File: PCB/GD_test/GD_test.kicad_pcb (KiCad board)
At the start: 2 copper layers, 46 x 51.3 mm, 47 parts, among them J1 RF_IN, J2 RF_IN, J3 RF_IN, J4 RF_IN, J5 Conn_01x01_Pin, J6 Conn_01x01_Pin, Q1 EPC2051, Q2 EPC2051, Q3 GS61004B-MR, Q5 EPC2014C, U1 LMG1020YFF, U10 TLV3501, U11 LMG1020YFF, U2 TLV3501, U3 NC7WZ04, U4 TLV3501, U5 NC7WZ04, U6 NC7WZ04, U7 NC7WZ04, U8 TLV3501, U9 LMG1020YFF

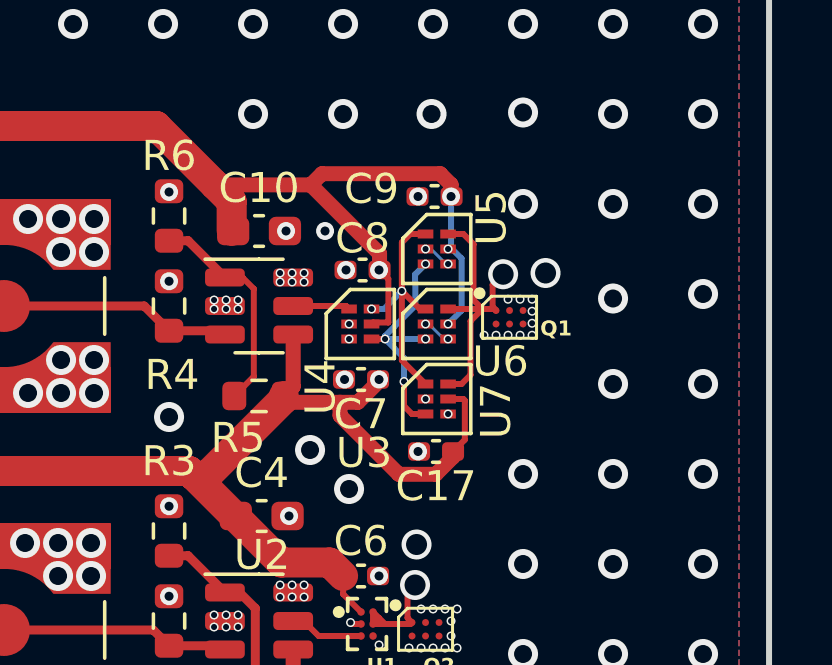
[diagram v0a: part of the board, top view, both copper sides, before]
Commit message: gate driver testboard rev 3 stuff
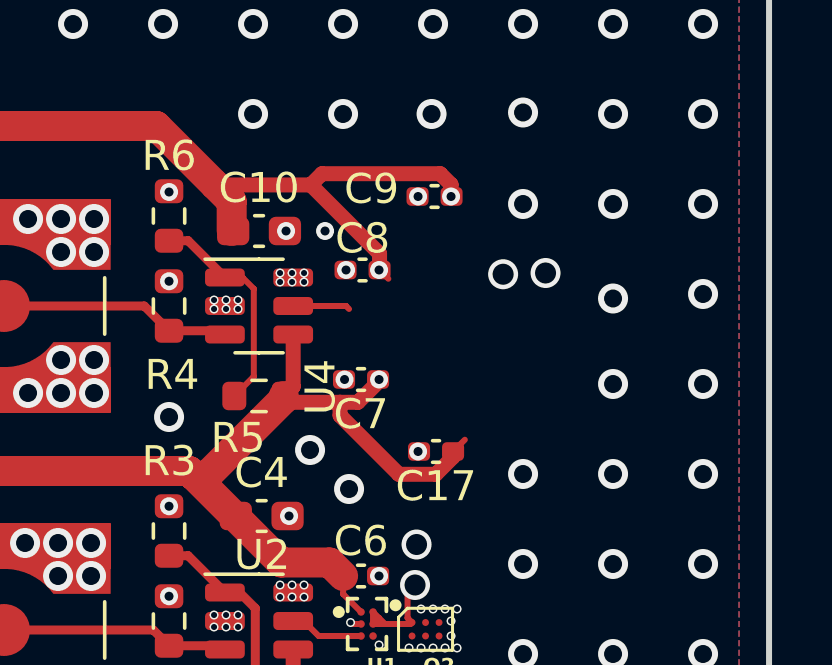
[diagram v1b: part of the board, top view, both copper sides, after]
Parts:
- removed Q1: EPC2051, EPCGaN:BGA-6_3x2_6.0x6.0mm
- removed U3, U5, U6, U7: NC7WZ04, pcbparts:SOIC-6
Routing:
- net Net-(Q1-G): track 9.54 -> 0.00 mm
- net +5V: track 186.2 -> 177.6 mm, vias 5 -> 3
- net /BUFF_OUT-: track 8.34 -> 0.00 mm, vias 4 -> 0
- net /BUFF_OUT+: track 8.25 -> 0.00 mm, vias 2 -> 0
- net GND: track 3.39 -> 1.47 mm, vias 368 -> 350

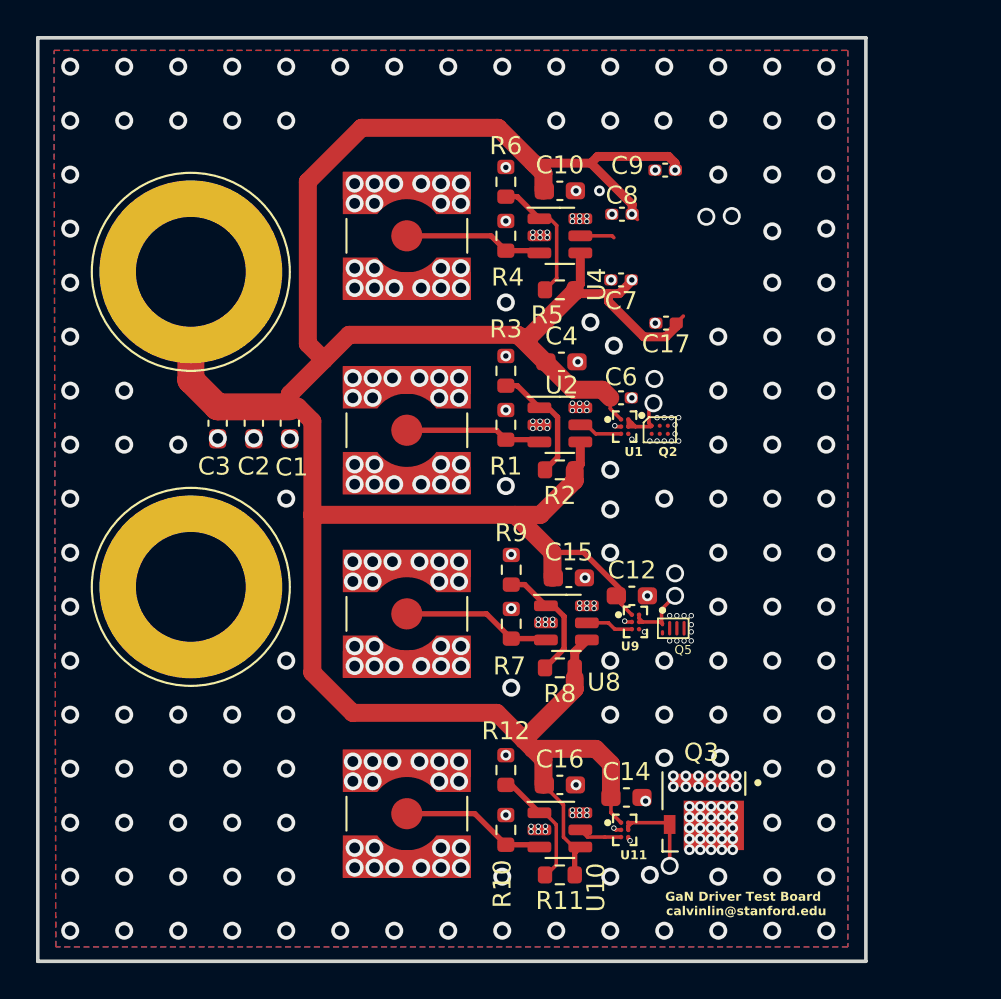
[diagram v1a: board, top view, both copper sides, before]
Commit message: gate driver test board rev 2 gerbers commit
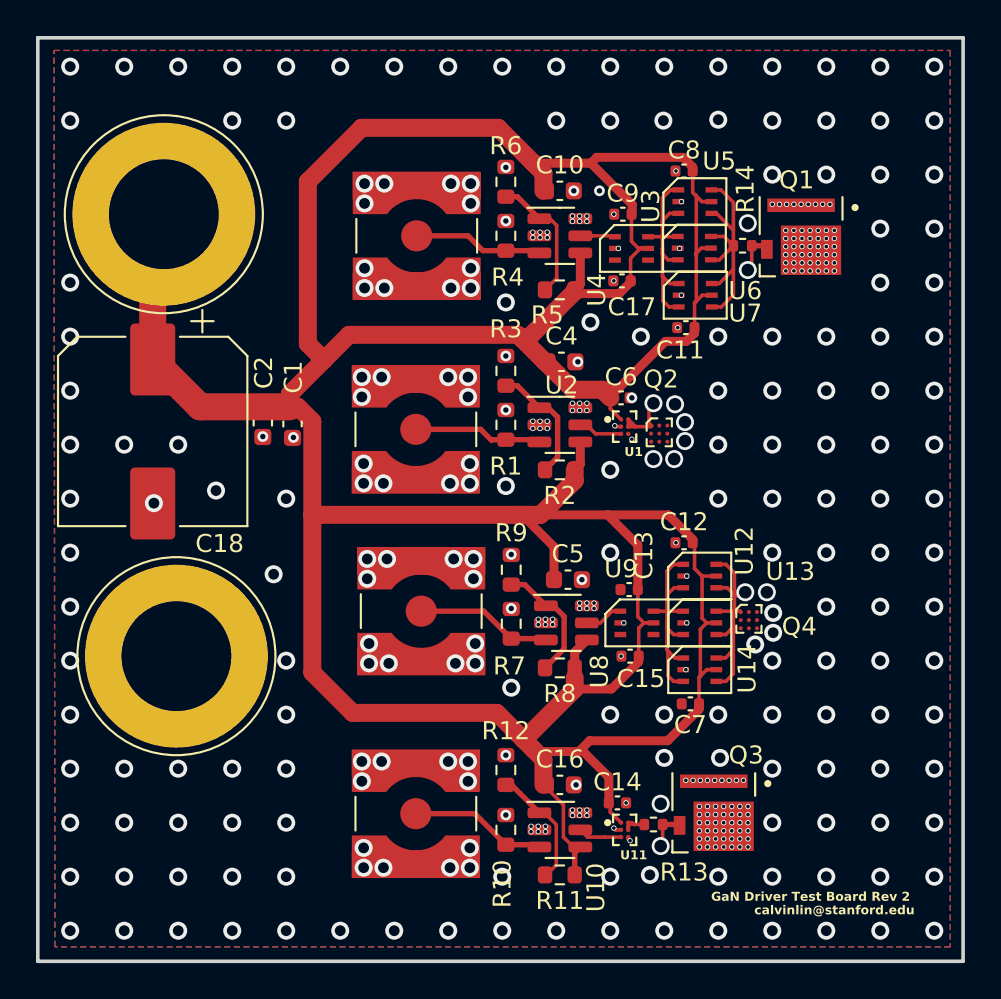
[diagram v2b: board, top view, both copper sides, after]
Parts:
- removed C3: C_Small, Capacitor_SMD:C_0603_1608Metric_Pad1.08x0.95mm_HandSolder
- removed Q5: EPC2014C, EPCGaN:EPC2014C
- added C11: C_Small, Capacitor_SMD:C_0402_1005Metric, F.Cu at (139.0, 81.6)
- added C13: C_Small, Capacitor_SMD:C_0402_1005Metric, F.Cu at (135.8, 96.2)
- added C18: C_Small, Capacitor_SMD:CP_Elec_10x10, F.Cu at (109.4, 87.4)
- added C5: C_Small, Capacitor_SMD:C_0603_1608Metric, F.Cu at (132.4, 95.6)
- added Q1: GS61004B-MR, EPCGaN:TRANS_GS61004B-MR, F.Cu at (145.4, 76.5)
- added Q4: EPC2214, pcbparts:BGA-9_3x3_6.0x6.0mm, F.Cu at (142.5, 97.8)
- added R13: 1, Resistor_SMD:R_0402_1005Metric, F.Cu at (137.2, 109.2)
- added R14: 1, Resistor_SMD:R_0402_1005Metric, F.Cu at (142.2, 77.0)
- added U12: NC7WZ04, pcbparts:nc7wz04_sc-88_SOIC-6, F.Cu at (139.8, 95.4)
- added U13: NC7WZ04, pcbparts:nc7wz04_sc-88_SOIC-6, F.Cu at (139.8, 98.0)
- added U14: NC7WZ04, pcbparts:nc7wz04_sc-88_SOIC-6, F.Cu at (139.8, 100.6)
- added U3: NC7WZ04, pcbparts:nc7wz04_sc-88_SOIC-6, F.Cu at (136.0, 77.2)
- added U5: NC7WZ04, pcbparts:nc7wz04_sc-88_SOIC-6, F.Cu at (139.5, 74.6)
- added U6: NC7WZ04, pcbparts:nc7wz04_sc-88_SOIC-6, F.Cu at (139.5, 77.2)
- added U7: NC7WZ04, pcbparts:nc7wz04_sc-88_SOIC-6, F.Cu at (139.5, 79.8)
- C1, C10, C16, C2, C4: footprint Capacitor_SMD:C_0603_1608Metric_Pad1.08x0.95mm_HandSolder -> Capacitor_SMD:C_0603_1608Metric
- C12, C14, C15: footprint Capacitor_SMD:C_0603_1608Metric_Pad1.08x0.95mm_HandSolder -> Capacitor_SMD:C_0402_1005Metric
- C17, C6, C7, C8, C9: footprint Capacitor_SMD:C_0402_1005Metric_Pad0.74x0.62mm_HandSolder -> Capacitor_SMD:C_0402_1005Metric
- Q2: value EPC2051 -> EPC2214; footprint EPCGaN:BGA-6_3x2_6.0x6.0mm -> pcbparts:BGA-9_3x3_6.0x6.0mm
- U9: value LMG1020YFF -> NC7WZ04; footprint GateDriver:BGA6N40P3X2_125X85X62N -> pcbparts:nc7wz04_sc-88_SOIC-6
- moved C7 23.9 mm to (139.2, 102.5)
- moved C15 5.52 mm to (135.9, 99.8)
- moved C8 4.20 mm to (138.9, 72.9), turned to 0 degrees
- moved C12 4.14 mm to (138.9, 93.5)
- moved J6 3.93 mm to (110.7, 99.8)
- moved J5 3.53 mm to (110.0, 75.3)
- moved C17 3.39 mm to (135.4, 79.0)
- moved C9 3.39 mm to (135.5, 75.3), turned to 0 degrees
- moved J2 0.81 mm to (124.3, 97.3)
- moved C14 0.58 mm to (135.2, 108.0)
- moved Q3 0.55 mm to (140.6, 108.5)
- moved J4 0.55 mm to (124.0, 76.5)
- moved J1 0.50 mm to (124.0, 87.2)
- moved C2 0.50 mm to (115.5, 86.9)
- moved J3 0.50 mm to (124.0, 108.6)
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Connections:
- C12 pad 1: +5V -> GND
- C12 pad 2: GND -> +5V
- C15 pad 1: +5V -> GND
- C15 pad 2: GND -> +5V
- C8 pad 1: +5V -> GND
- C8 pad 2: GND -> +5V
- C9 pad 1: +5V -> GND
- C9 pad 2: GND -> +5V
- Q3 pad 2: Net-(U11-OUTH) -> Net-(Q3-Pad2)
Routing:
- net +5V: track 177.6 -> 229.9 mm, vias 3 -> 0
- net Net-(U5-Y1): track 0.00 -> 14.3 mm
- net Net-(Q4-G): track 0.00 -> 13.8 mm, vias 0 -> 1
- net Net-(U3-Y1): track 0.00 -> 13.2 mm
- net /inv_out: track 0.00 -> 13.0 mm
- net Net-(U11-OUTH): track 5.52 -> 1.81 mm, vias 1 -> 0
- net Net-(Q5-G): track 3.70 -> 0.00 mm, vias 1 -> 0
- net Net-(Q1-Pad2): track 0.00 -> 2.36 mm, vias 0 -> 1
- net Net-(Q3-Pad2): track 0.00 -> 2.28 mm, vias 0 -> 1
- net /RF_IN_3: track 8.33 -> 7.59 mm
- net Net-(U3-A1): track 1.90 -> 2.57 mm
- net /RF_IN_2: track 7.76 -> 7.21 mm
- net Net-(U8-OUT): track 2.64 -> 2.13 mm
- net /RF_IN_4: track 8.13 -> 7.63 mm
- net GND: track 1.47 -> 1.05 mm, vias 350 -> 392
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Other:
- board size 46 x 51.3 mm -> 51.4 x 51.3 mm
- board text added: "GaN Driver Test Board Rev 2"
- board text removed: "GaN Driver Test Board"
